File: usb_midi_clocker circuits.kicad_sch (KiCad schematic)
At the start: 25 parts, among them J1 SD card breakout, J2 USB power, J3 PJS008U-3000-0, J4 USB Host header, J5 Conn_01x08_Pin, SW1 Rotary_Encoder_Switch, SW2 SW_Push_Back, SW3 SW_Push_Select, U1 L78L05_TO92, U2 Teensy4.1, U3 TFT_320x240

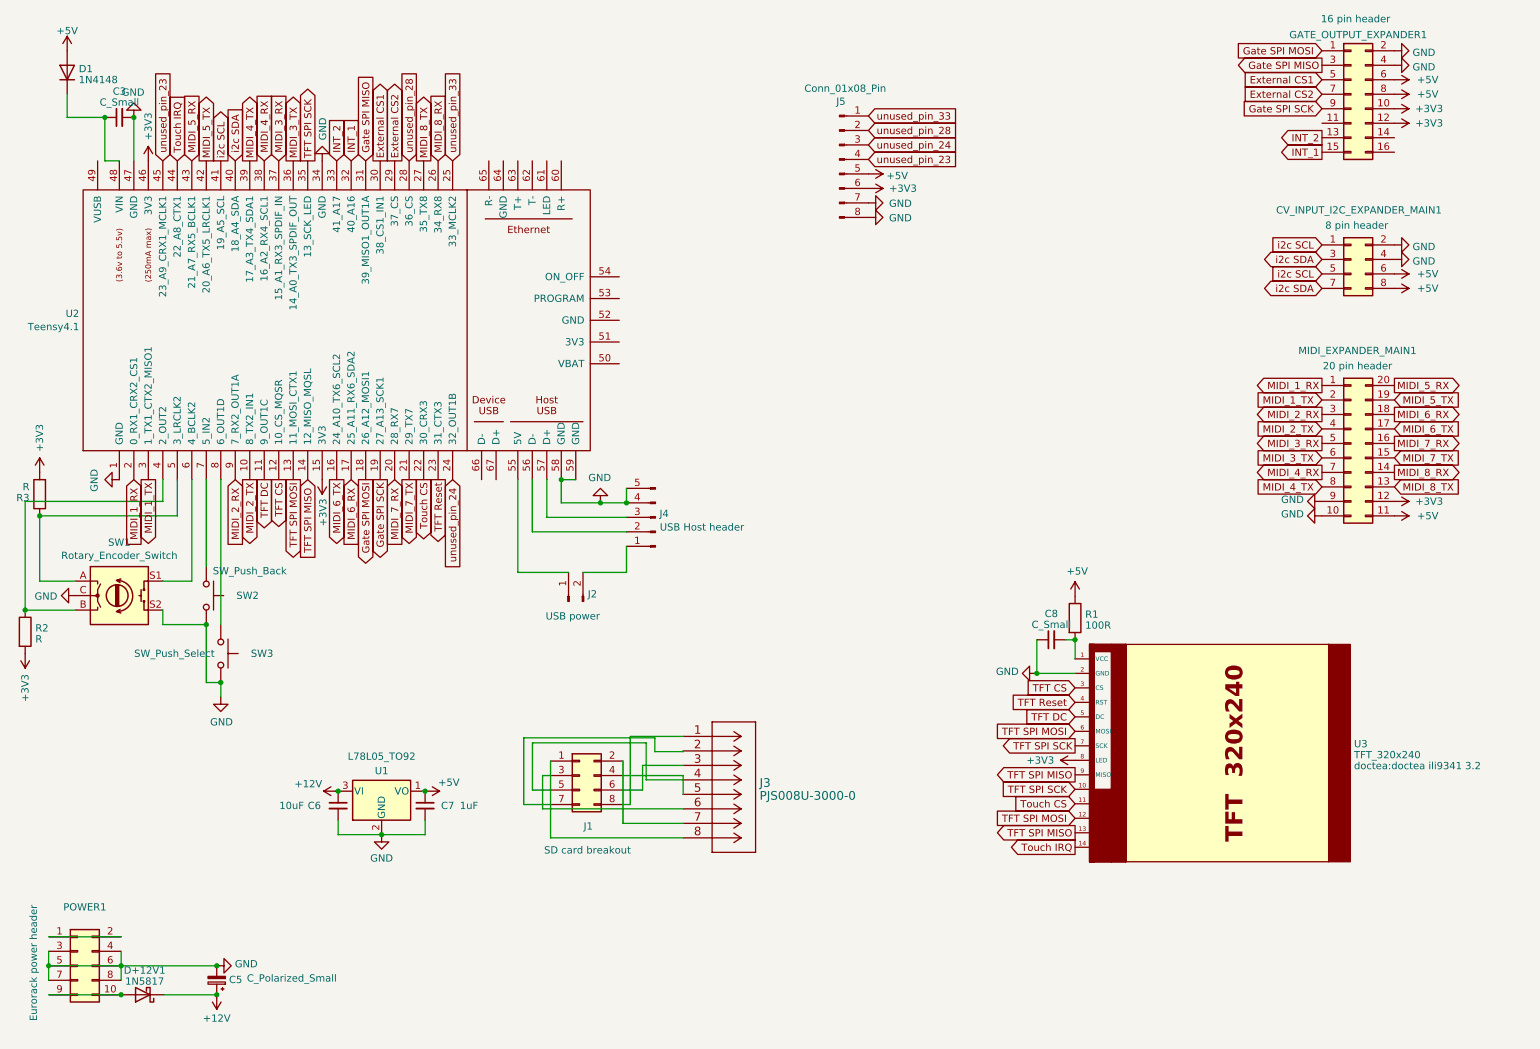
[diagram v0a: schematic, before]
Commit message: laid out
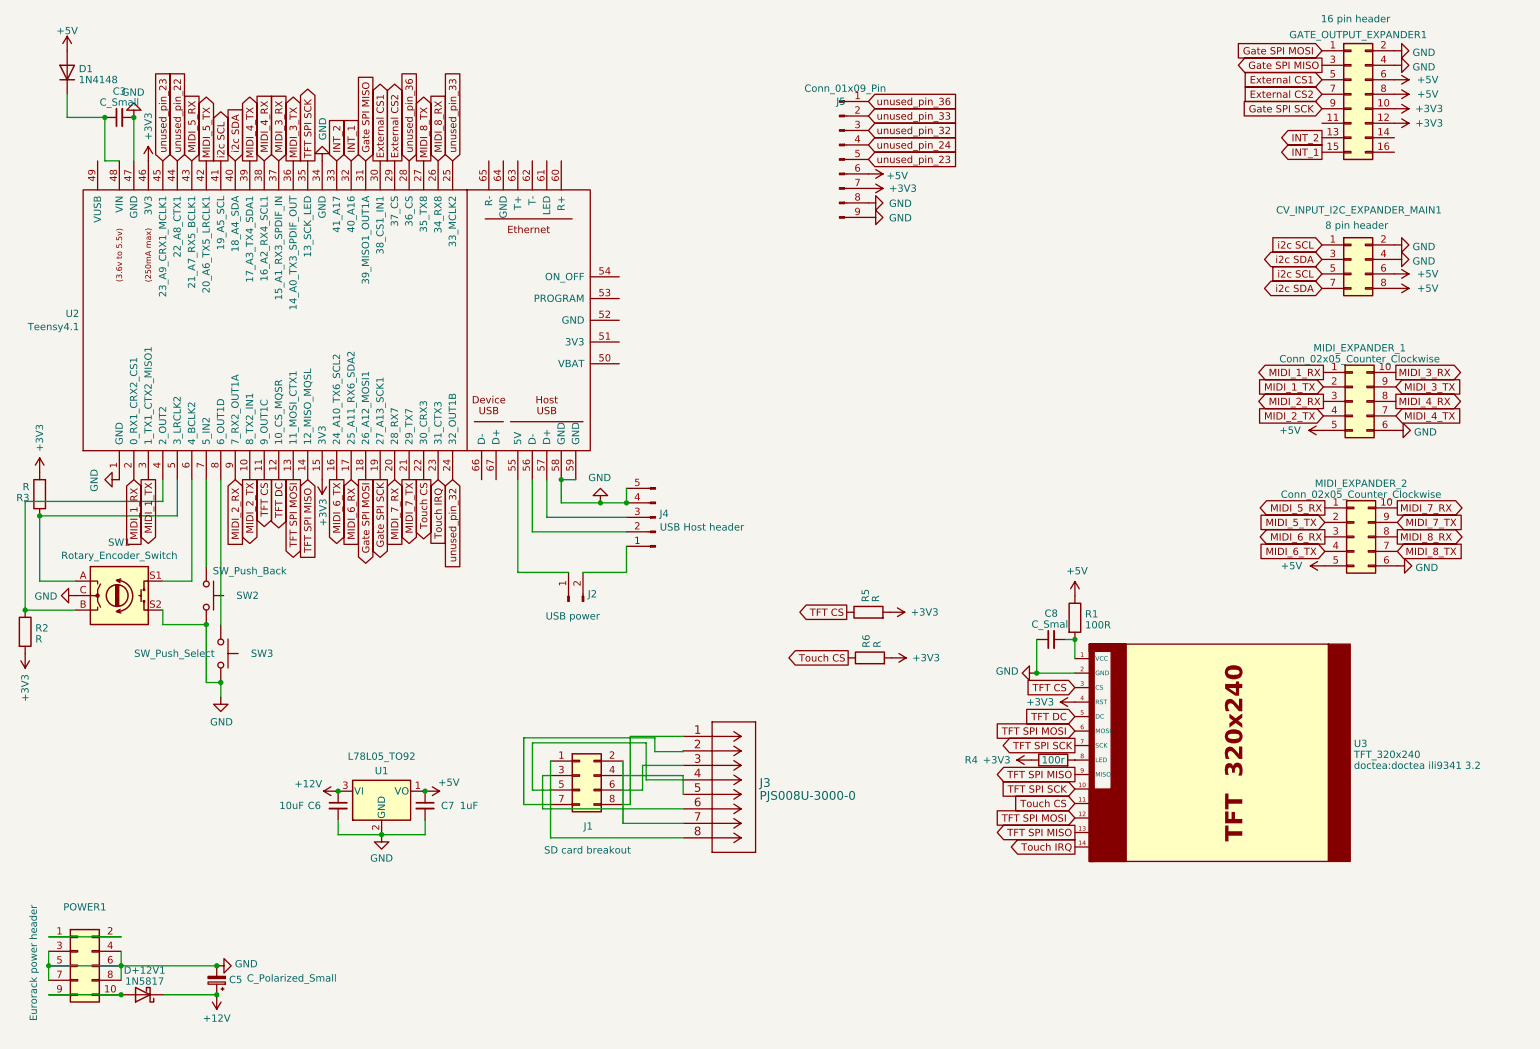
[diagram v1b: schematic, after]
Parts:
- removed MIDI_EXPANDER_MAIN1: 20 pin header, Connector_PinHeader_2.54mm:PinHeader_2x10_P2.54mm_Vertical, symbol Connector_Generic:Conn_02x10_Counter_Clockwise
- added MIDI_EXPANDER_1, MIDI_EXPANDER_2: Conn_02x05_Counter_Clockwise, Connector_PinHeader_2.54mm:PinHeader_2x05_P2.54mm_Vertical, symbol Connector_Generic:Conn_02x05_Counter_Clockwise
- added R4: 100r, Resistor_THT:R_Axial_DIN0309_L9.0mm_D3.2mm_P2.54mm_Vertical, symbol Device:R
- added R5, R6: R, Resistor_THT:R_Axial_DIN0309_L9.0mm_D3.2mm_P2.54mm_Vertical, symbol Device:R
- J5: value Conn_01x08_Pin -> Conn_01x09_Pin; footprint doctea:PinHeader_2x04_P2.54mm_Vertical-AlternatePinNumbering -> doctea:PinHeader_2x05_P2.54mm_Vertical-AlternatePinNumbering; symbol Connector:Conn_01x08_Pin -> Connector:Conn_01x09_Pin
- R1: footprint Resistor_THT:R_Axial_DIN0207_L6.3mm_D2.5mm_P10.16mm_Horizontal -> Resistor_THT:R_Axial_DIN0309_L9.0mm_D3.2mm_P2.54mm_Vertical
- R2, R3: footprint (none) -> Resistor_THT:R_Axial_DIN0309_L9.0mm_D3.2mm_P2.54mm_Vertical
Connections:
- net +3V3: now also J5.7 (Pin_7), U3.4 (RST), R4.1, R5.2, R6.2; no longer J5.6 (Pin_6), U3.8 (LED)
- net +5V: now also J5.6 (Pin_6), MIDI_EXPANDER_1.5 (Pin_5), MIDI_EXPANDER_2.5 (Pin_5); no longer J5.5 (Pin_5)
- net GND: now also J5.9 (Pin_9), MIDI_EXPANDER_1.6 (Pin_6), MIDI_EXPANDER_2.6 (Pin_6); no longer J5.7 (Pin_7)
- net MIDI_1_RX: now also MIDI_EXPANDER_1.1 (Pin_1)
- net MIDI_1_TX: now also MIDI_EXPANDER_1.2 (Pin_2)
- net MIDI_2_RX: now also MIDI_EXPANDER_1.3 (Pin_3)
- net MIDI_2_TX: now also MIDI_EXPANDER_1.4 (Pin_4)
- net MIDI_3_RX: now also MIDI_EXPANDER_1.10 (Pin_10)
- net MIDI_3_TX: now also MIDI_EXPANDER_1.9 (Pin_9)
- net MIDI_4_RX: now also MIDI_EXPANDER_1.8 (Pin_8)
- net MIDI_4_TX: now also MIDI_EXPANDER_1.7 (Pin_7)
- net MIDI_5_RX: now also MIDI_EXPANDER_2.1 (Pin_1)
- net MIDI_5_TX: now also MIDI_EXPANDER_2.2 (Pin_2)
- net MIDI_6_RX: now also MIDI_EXPANDER_2.3 (Pin_3)
- net MIDI_6_TX: now also MIDI_EXPANDER_2.4 (Pin_4)
- net MIDI_7_RX: now also MIDI_EXPANDER_2.10 (Pin_10)
- net MIDI_7_TX: now also MIDI_EXPANDER_2.9 (Pin_9)
- net MIDI_8_RX: now also MIDI_EXPANDER_2.8 (Pin_8)
- net MIDI_8_TX: now also MIDI_EXPANDER_2.7 (Pin_7)
- net TFT CS: now also U2.11 (9_OUT1C), R5.1; no longer U2.12 (10_CS_MQSR)
- net TFT DC: now also U2.12 (10_CS_MQSR); no longer U2.11 (9_OUT1C)
- net Touch CS: now also R6.1
- net Touch IRQ: now also U2.23 (31_CTX3); no longer U2.44 (22_A8_CTX1)
- net unused_pin_23: now also J5.5 (Pin_5); no longer J5.4 (Pin_4)
- net unused_pin_24: now also J5.4 (Pin_4); no longer J5.3 (Pin_3), U2.24 (32_OUT1B)
- net unused_pin_33: now also J5.2 (Pin_2); no longer J5.1 (Pin_1)
- removed net TFT Reset: U2.23 (31_CTX3), U3.4 (RST)
- net unused_pin_28 renamed unused_pin_36
- net unused_pin_36: now also J5.1 (Pin_1); no longer J5.2 (Pin_2)
- new net: R4.2, U3.8 (LED)
- new net unused_pin_22: U2.44 (22_A8_CTX1)
- new net unused_pin_32: J5.3 (Pin_3), U2.24 (32_OUT1B)

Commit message: laid out some more
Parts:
- J5: footprint doctea:PinHeader_2x05_P2.54mm_Vertical-AlternatePinNumbering -> doctea:PinHeader_2x05_P2.54mm_Vertical
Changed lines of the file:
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@@
       (effects (font (size 1.27 1.27)))
     )
-    (property "Footprint" "doctea:PinHeader_2x05_P2.54mm_Vertical-AlternatePinNumbering" (at 164.846 40.894 0)
+    (property "Footprint" "doctea:PinHeader_2x05_P2.54mm_Vertical" (at 164.846 40.894 0)
       (effects (font (size 1.27 1.27)) hide)
     )

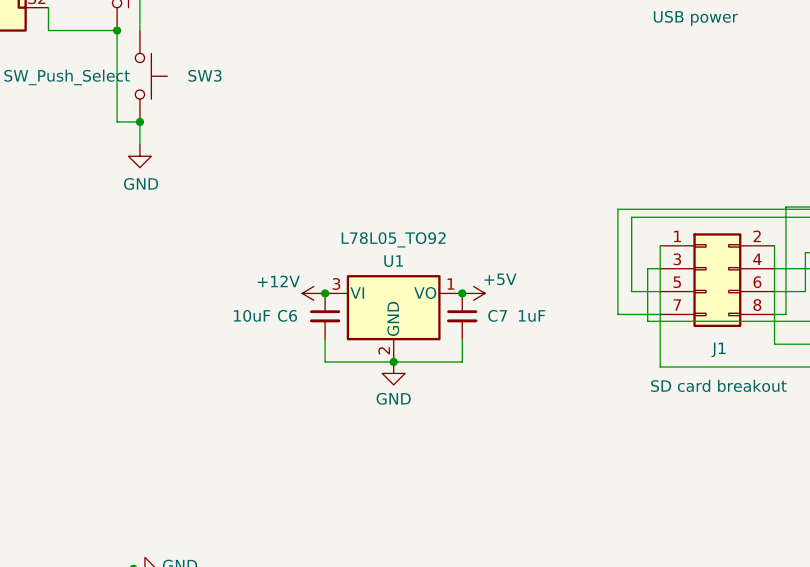
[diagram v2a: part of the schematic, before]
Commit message: solve a couple of problems on main board + main panel
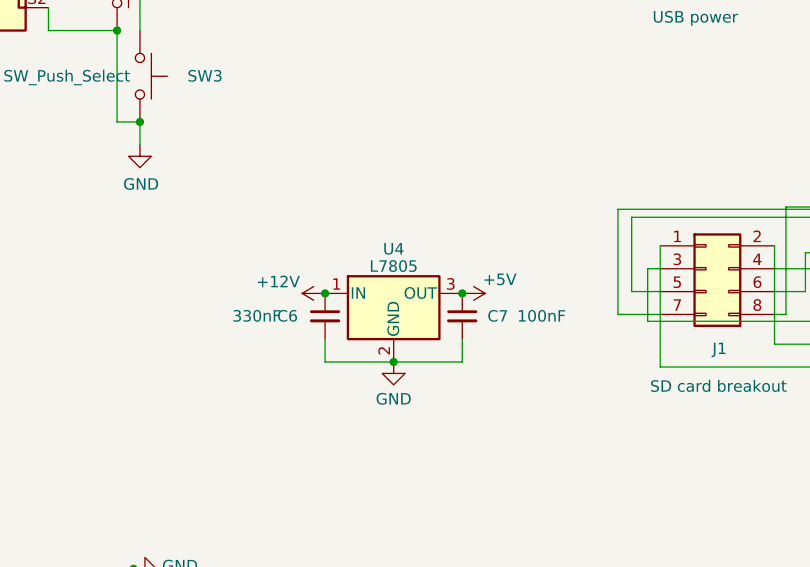
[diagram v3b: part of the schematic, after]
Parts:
- removed U1: L78L05_TO92, Package_TO_SOT_THT:TO-92_Inline, symbol Regulator_Linear:L78L05_TO92
- added U4: L7805, Package_TO_SOT_THT:TO-220-3_Vertical, symbol Regulator_Linear:L7805
- C6: value 10uF -> 330nF
- C7: value 1uF -> 100nF
- J5: footprint doctea:PinHeader_2x05_P2.54mm_Vertical -> Connector_PinHeader_2.54mm:PinHeader_2x05_P2.54mm_Vertical
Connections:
- net +12V: now also U4.1 (IN)
- net +5V: now also U4.3 (OUT)
- net GND: now also U4.2 (GND)
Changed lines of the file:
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@@
   (junction (at 55.6768 187.325) (diameter 0) (color 0 0 0 0)
   )
+  (junction (at 92.202 151.638) (diameter 0) (color 0 0 0 0)
+  )
   (junction (at 116.078 97.028) (diameter 0) (color 0 0 0 0)
   )
+  (junction (at 22.098 119.888) (diameter 0) (color 0 0 0 0)
+  )
+  (junction (at 38.9128 182.245) (diameter 0) (color 0 0 0 0)
+  )
+  (junction (at 41.148 33.528) (diameter 0) (color 0 0 0 0)
+  )
+  (junction (at 24.638 103.378) (diameter 0) (color 0 0 0 0)
+  )
+  (junction (at 53.848 122.428) (diameter 0) (color 0 0 0 0)
+  )
+  (junction (at 36.068 33.528) (diameter 0) (color 0 0 0 0)
+  )
+  (junction (at 206.121 125.0442) (diameter 0) (color 0 0 0 0)
+  )
+  (junction (at 56.388 132.588) (diameter 0) (color 0 0 0 0)
+  )
+  (junction (at 38.9128 187.325) (diameter 0) (color 0 0 0 0)
+  )
+  (junction (at 122.936 101.092) (diameter 0) (color 0 0 0 0)
+  )
+  (junction (at 55.6768 182.245) (diameter 0) (color 0 0 0 0)
+  )
+  (junction (at 127.508 101.092) (diameter 0) (color 0 0 0 0)
+  )
+  (junction (at 84.582 159.258) (diameter 0) (color 0 0 0 0)
+  )
+  (junction (at 199.4154 130.937) (diameter 0) (color 0 0 0 0)
+  )
   (junction (at 76.962 151.638) (diameter 0) (color 0 0 0 0)
-  )
-  (junction (at 22.098 119.888) (diameter 0) (color 0 0 0 0)
-  )
-  (junction (at 38.9128 182.245) (diameter 0) (color 0 0 0 0)
-  )
-  (junction (at 92.202 151.638) (diameter 0) (color 0 0 0 0)
-  )
-  (junction (at 41.148 33.528) (diameter 0) (color 0 0 0 0)
-  )
-  (junction (at 24.638 103.378) (diameter 0) (color 0 0 0 0)
-  )
-  (junction (at 53.848 122.428) (diameter 0) (color 0 0 0 0)
-  )
-  (junction (at 36.068 33.528) (diameter 0) (color 0 0 0 0)
-  )
-  (junction (at 206.121 125.0442) (diameter 0) (color 0 0 0 0)
-  )
-  (junction (at 56.388 132.588) (diameter 0) (color 0 0 0 0)
-  )
-  (junction (at 38.9128 187.325) (diameter 0) (color 0 0 0 0)
-  )
-  (junction (at 122.936 101.092) (diameter 0) (color 0 0 0 0)
-  )
-  (junction (at 55.6768 182.245) (diameter 0) (color 0 0 0 0)
-  )
-  (junction (at 127.508 101.092) (diameter 0) (color 0 0 0 0)
-  )
-  (junction (at 84.582 159.258) (diameter 0) (color 0 0 0 0)
-  )
-  (junction (at 199.4154 130.937) (diameter 0) (color 0 0 0 0)
   )
   (junction (at 26.2128 182.245) (diameter 0) (color 0 0 0 0)
@@
       (effects (font (size 1.27 1.27)) (justify left))
     )
-    (property "Value" "10uF" (at 66.6496 154.178 0)
+    (property "Value" "330nF" (at 66.6496 154.178 0)
       (effects (font (size 1.27 1.27)) (justify left))
     )
@@
     )
   )
-  (symbol (lib_id "Regulator_Linear:L78L05_TO92") (at 84.582 151.638 0) (unit 1)
-    (in_bom yes) (on_board yes) (dnp no)
-    (property "Reference" "U1" (at 84.582 148.082 0)
-      (effects (font (size 1.27 1.27)))
-    )
-    (property "Value" "L78L05_TO92" (at 84.582 145.542 0)
-      (effects (font (size 1.27 1.27)))
-    )
-    (property "Footprint" "Package_TO_SOT_THT:TO-92_Inline" (at 84.582 145.923 0)
-      (effects (font (size 1.27 1.27) italic) hide)
-    )
-    (property "Datasheet" "http://www.st.com/content/ccc/resource/technical/document/datasheet/15/55/e5/aa/23/5b/43/fd/CD00000446.pdf/files/CD00000446.pdf/jcr:content/translations/en.CD00000446.pdf" (at 84.582 152.908 0)
-      (effects (font (size 1.27 1.27)) hide)
-    )
-    (pin "1")
-    (pin "2")
-    (pin "3")
-    (instances
-      (project "usb_midi_clocker circuits"
-        (path "/34c98e31-06d2-46ec-970e-3acc65b5aead"
-          (reference "U1") (unit 1)
-        )
-      )
-    )
-  )
   (symbol (lib_id "power:+3V3") (at 24.638 95.758 0) (unit 1)
     (in_bom yes) (on_board yes) (dnp no)
@@
     )
   )
+  (symbol (lib_id "Regulator_Linear:L7805") (at 84.582 151.638 0) (unit 1)
+    (in_bom yes) (on_board yes) (dnp no) (fields_autoplaced)
+    (property "Reference" "U4" (at 84.582 146.7231 0)
+      (effects (font (size 1.27 1.27)))
+    )
+    (property "Value" "L7805" (at 84.582 148.6441 0)
+      (effects (font (size 1.27 1.27)))
+    )
+    (property "Footprint" "Package_TO_SOT_THT:TO-220-3_Vertical" (at 85.217 155.448 0)
+      (effects (font (size 1.27 1.27) italic) (justify left) hide)
+    )
+    (property "Datasheet" "http://www.st.com/content/ccc/resource/technical/document/datasheet/41/4f/b3/b0/12/d4/47/88/CD00000444.pdf/files/CD00000444.pdf/jcr:content/translations/en.CD00000444.pdf" (at 84.582 152.908 0)
+      (effects (font (size 1.27 1.27)) hide)
+    )
+    (pin "1")
+    (pin "2")
+    (pin "3")
+    (instances
+      (project "usb_midi_clocker circuits"
+        (path "/34c98e31-06d2-46ec-970e-3acc65b5aead"
+          (reference "U4") (unit 1)
+        )
+      )
+    )
+  )
   (symbol (lib_id "power:+3V3") (at 74.168 97.028 180) (unit 1)
     (in_bom yes) (on_board yes) (dnp no)
@@
       (effects (font (size 1.27 1.27)))
     )
-    (property "Footprint" "doctea:PinHeader_2x05_P2.54mm_Vertical" (at 164.846 40.894 0)
+    (property "Footprint" "Connector_PinHeader_2.54mm:PinHeader_2x05_P2.54mm_Vertical" (at 164.846 40.894 0)
       (effects (font (size 1.27 1.27)) hide)
     )
@@
       (effects (font (size 1.27 1.27)) (justify left))
     )
-    (property "Value" "1uF" (at 98.298 154.178 0)
+    (property "Value" "100nF" (at 98.298 154.178 0)
       (effects (font (size 1.27 1.27)) (justify left))
     )
